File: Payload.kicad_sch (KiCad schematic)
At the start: 1 part, among them U1 STM32-(STM32H745ZIT6)

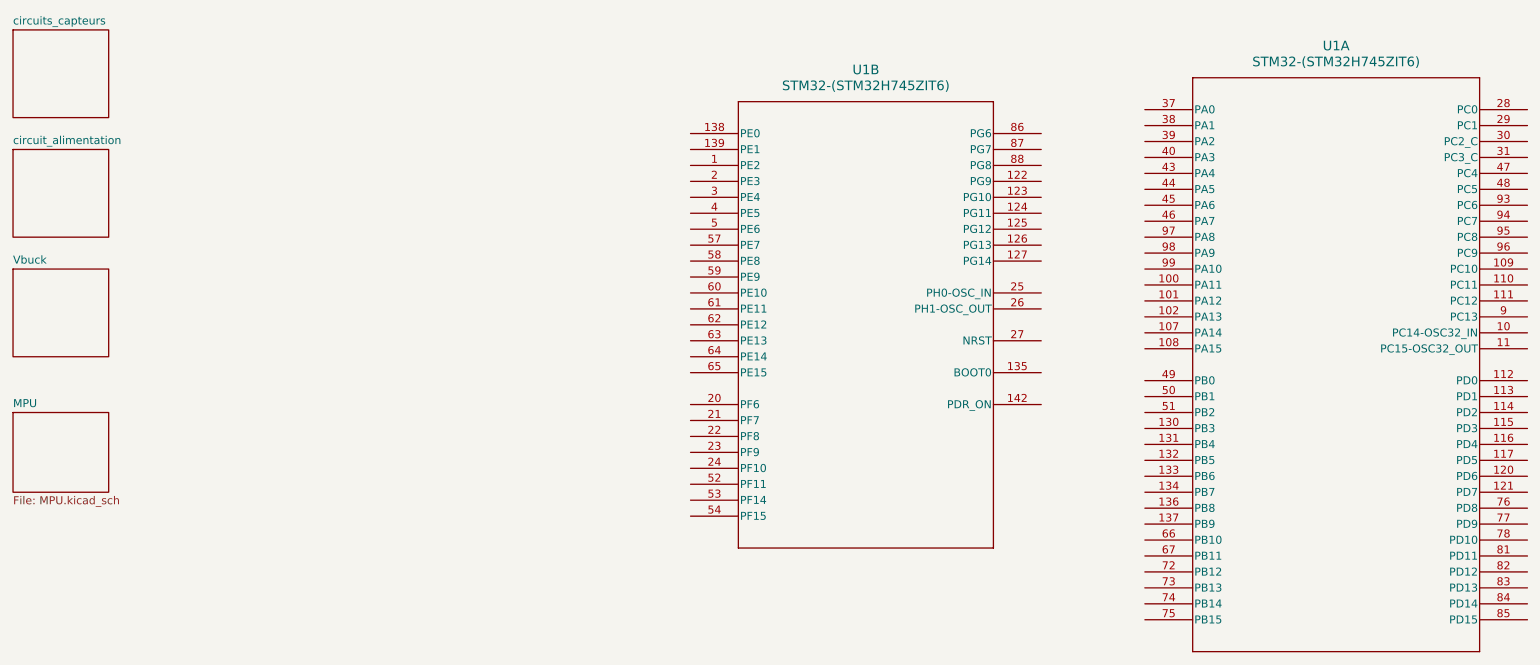
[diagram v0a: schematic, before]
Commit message: Revert "Recommit du Vbuck"
This reverts commit db6b1385e92bec759ec8c6f30127fdc08b8b4918.
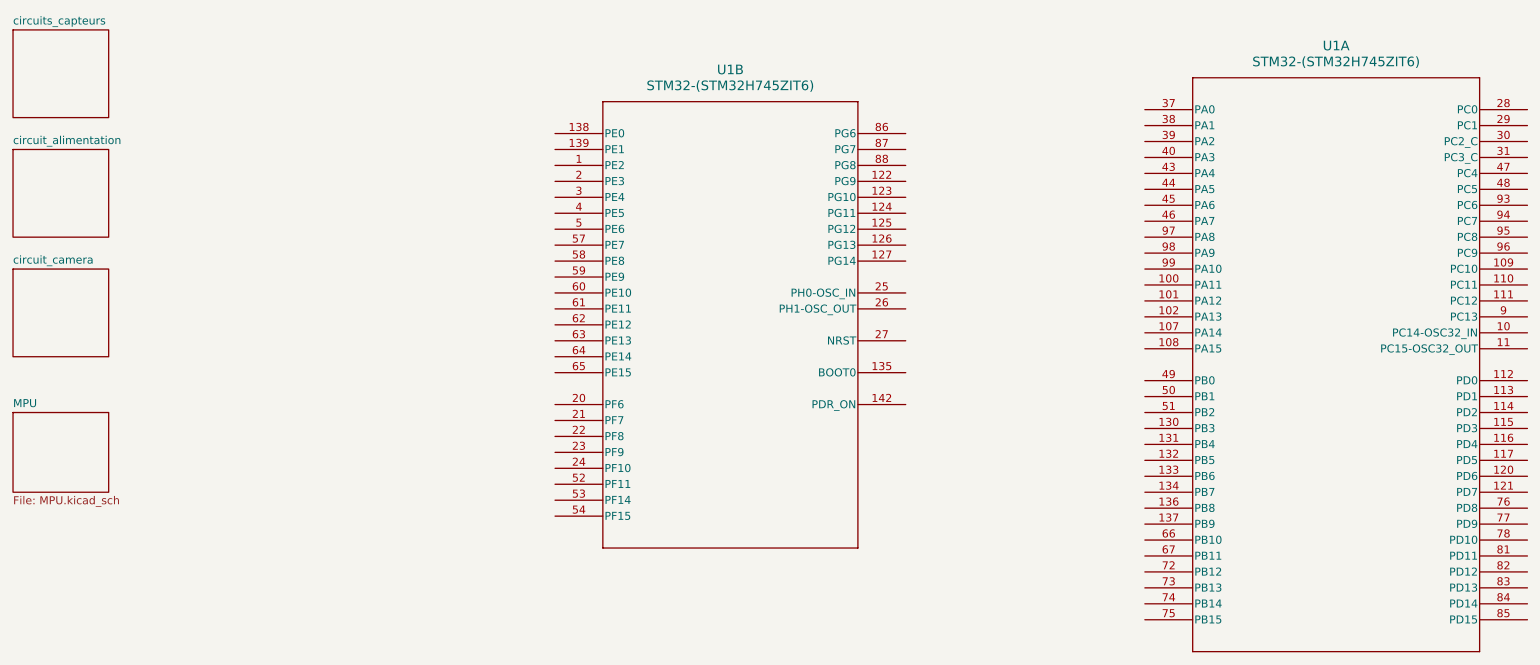
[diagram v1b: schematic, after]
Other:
- sheet Vbuck renamed circuit_camera
- moved on the sheet: U1B
